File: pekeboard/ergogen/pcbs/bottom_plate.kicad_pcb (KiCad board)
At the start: 2 copper layers, 156.8 x 132.1 mm, 0 parts

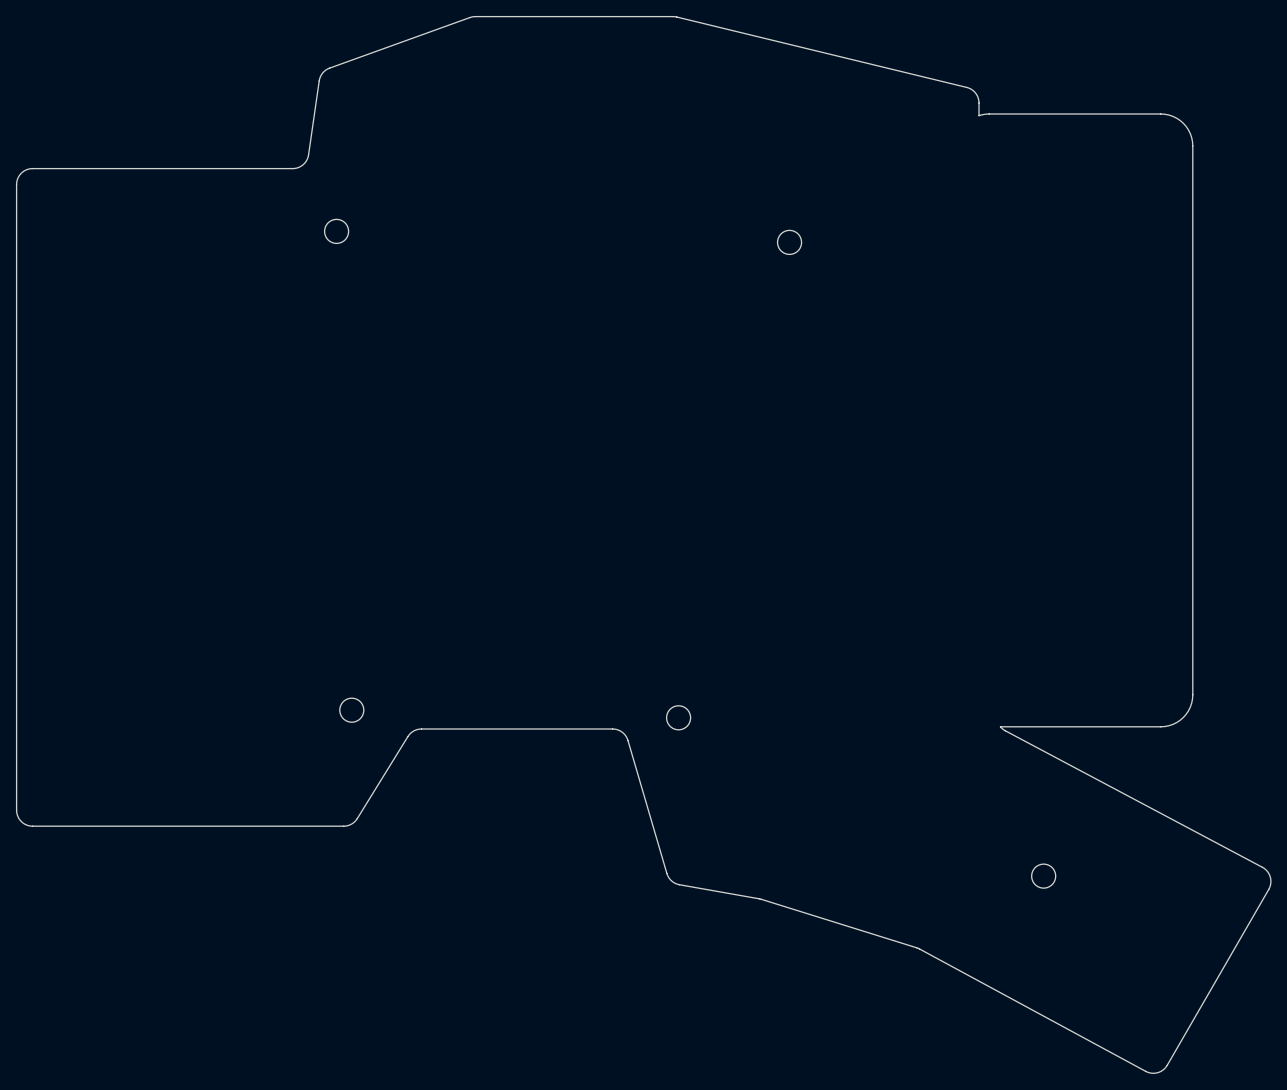
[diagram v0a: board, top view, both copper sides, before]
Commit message: Extreme trimming
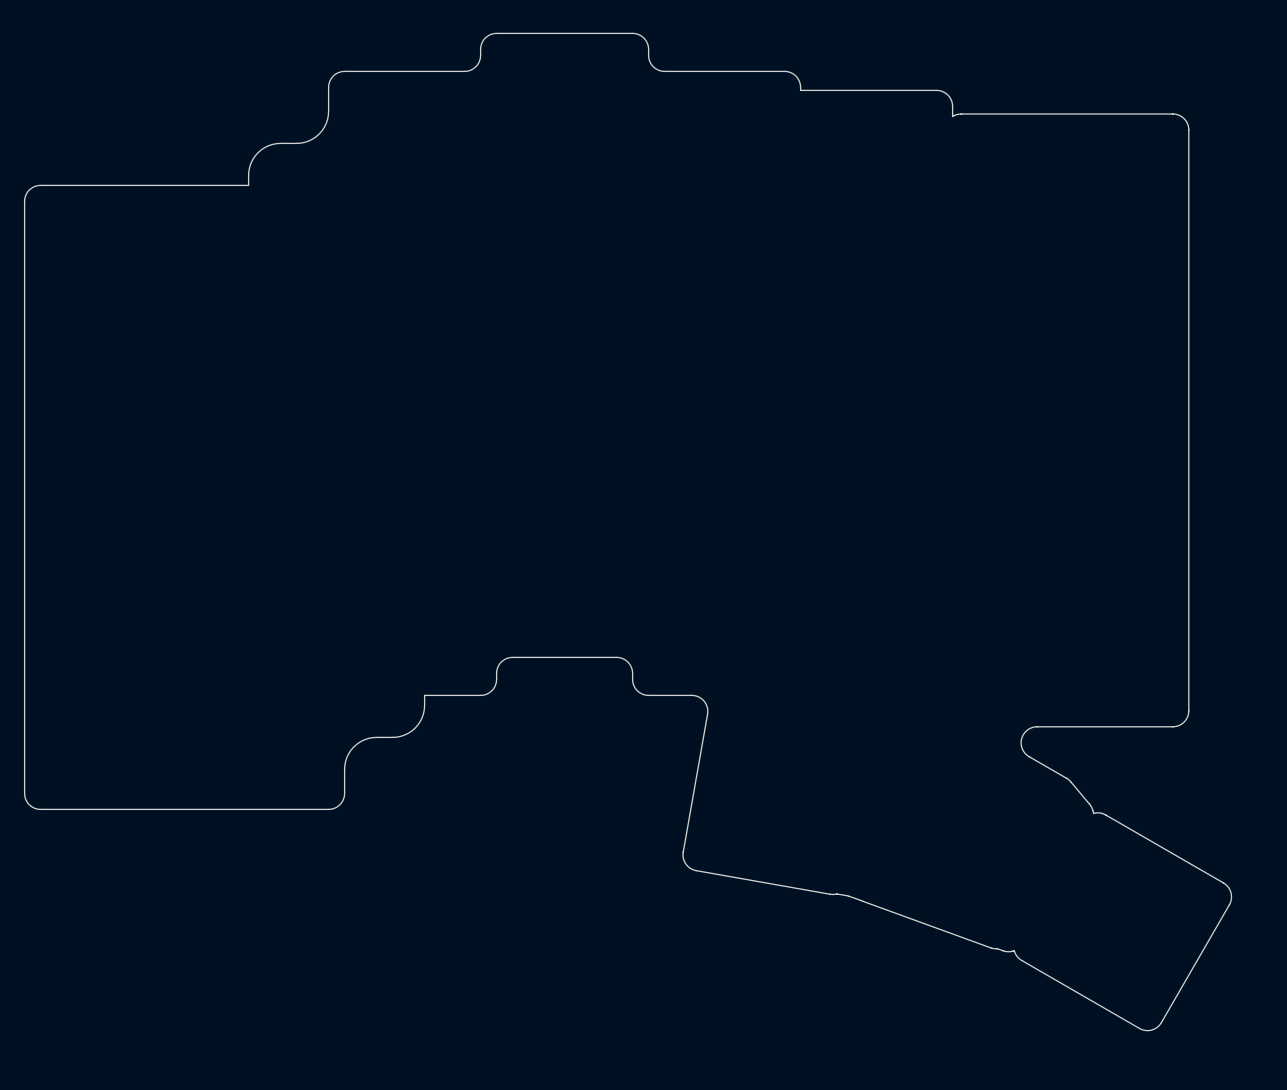
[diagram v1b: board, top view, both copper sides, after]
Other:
- board size 156.8 x 132.1 mm -> 150.9 x 124.7 mm
